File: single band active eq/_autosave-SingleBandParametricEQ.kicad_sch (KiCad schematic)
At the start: 18 parts, among them U1 TL081, U2 TL084

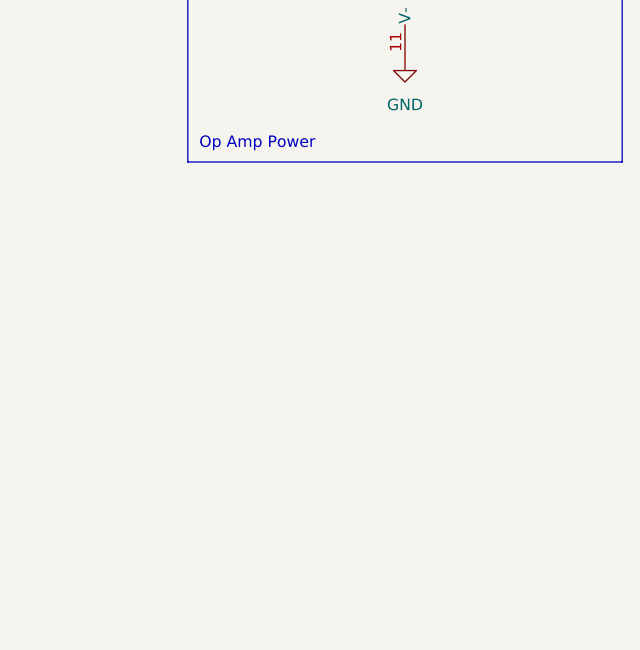
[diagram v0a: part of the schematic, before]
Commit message: Updated README
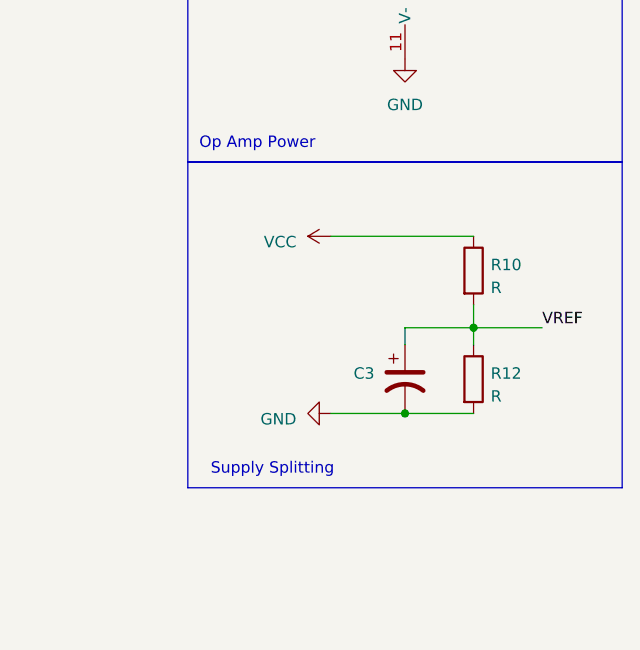
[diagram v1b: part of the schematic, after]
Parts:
- added C3: C_Polarized_US, symbol Device:C_Polarized_US
- added R10, R12: R, symbol Device:R
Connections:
- net GND: now also C3.2, R12.2
- net VCC: now also R10.1
- net VREF: now also C3.1, R10.2, R12.1
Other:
- note added: "Supply Splitting"
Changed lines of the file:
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@@
   (junction (at 53.975 46.99) (diameter 0) (color 0 0 0 0)
   )
+  (junction (at 268.605 69.85) (diameter 0) (color 0 0 0 0)
+  )
   (junction (at 173.99 54.61) (diameter 0) (color 0 0 0 0)
   )
@@
   (junction (at 43.18 124.46) (diameter 0) (color 0 0 0 0)
   )
+  (junction (at 260.985 79.375) (diameter 0) (color 0 0 0 0)
+  )
   (wire (pts (xy 66.04 63.5) (xy 112.395 63.5))
     (stroke (width 0) (type default))
@@
     (stroke (width 0) (type default))
   )
+  (wire (pts (xy 260.985 69.85) (xy 260.985 71.755))
+    (stroke (width 0) (type default))
+  )
   (wire (pts (xy 112.395 63.5) (xy 158.75 63.5))
     (stroke (width 0) (type default))
@@
     (stroke (width 0) (type default))
   )
+  (wire (pts (xy 260.985 69.85) (xy 268.605 69.85))
+    (stroke (width 0) (type default))
+  )
   (wire (pts (xy 92.71 41.91) (xy 92.71 49.53))
     (stroke (width 0) (type default))
@@
     (stroke (width 0) (type default))
   )
+  (wire (pts (xy 252.73 59.69) (xy 268.605 59.69))
+    (stroke (width 0) (type default))
+  )
   (wire (pts (xy 32.385 40.64) (xy 32.385 46.99))
     (stroke (width 0) (type default))
@@
     (stroke (width 0) (type default))
   )
+  (wire (pts (xy 260.985 79.375) (xy 268.605 79.375))
+    (stroke (width 0) (type default))
+  )
   (wire (pts (xy 76.2 111.76) (xy 76.2 127))
     (stroke (width 0) (type default))
@@
     (stroke (width 0) (type default))
   )
+  (wire (pts (xy 268.605 67.31) (xy 268.605 69.85))
+    (stroke (width 0) (type default))
+  )
   (wire (pts (xy 83.82 73.66) (xy 83.82 87.63))
     (stroke (width 0) (type default))
@@
     (stroke (width 0) (type default))
   )
+  (wire (pts (xy 268.605 69.85) (xy 276.225 69.85))
+    (stroke (width 0) (type default))
+  )
   (wire (pts (xy 101.6 85.09) (xy 104.14 85.09))
     (stroke (width 0) (type default))
@@
     (stroke (width 0) (type default))
   )
+  (wire (pts (xy 268.605 69.85) (xy 268.605 71.755))
+    (stroke (width 0) (type default))
+  )
   (wire (pts (xy 127.635 85.09) (xy 144.145 85.09))
     (stroke (width 0) (type default))
@@
     (stroke (width 0) (type default))
   )
+  (wire (pts (xy 260.985 79.375) (xy 252.73 79.375))
+    (stroke (width 0) (type default))
+  )
   (wire (pts (xy 137.16 52.07) (xy 138.43 52.07))
     (stroke (width 0) (type default))
@@
   )
   (rectangle (start 236.855 12.065) (end 285.115 51.435)
+    (stroke (width 0) (type default))
+    (fill (type none))
+  )
+  (rectangle (start 236.855 51.435) (end 285.115 87.63)
     (stroke (width 0) (type default))
     (fill (type none))
@@
   )
   (text "Cut/Boost Stage\n" (at 13.97 163.83 0)
+    (effects (font (size 1.27 1.27)) (justify left bottom))
+  )
+  (text "Supply Splitting\n" (at 239.395 86.36 0)
+    (effects (font (size 1.27 1.27)) (justify left bottom))
+  )
+  (label "VREF" (at 276.225 69.85 0) (fields_autoplaced)
     (effects (font (size 1.27 1.27)) (justify left bottom))
   )
@@
     )
   )
+  (symbol (lib_id "Device:R") (at 268.605 75.565 0) (unit 1)
+    (in_bom yes) (on_board yes) (dnp no) (fields_autoplaced)
+    (property "Reference" "R12" (at 270.51 74.93 0)
+      (effects (font (size 1.27 1.27)) (justify left))
+    )
+    (property "Value" "R" (at 270.51 77.47 0)
+      (effects (font (size 1.27 1.27)) (justify left))
+    )
+    (property "Footprint" "" (at 266.827 75.565 90)
+      (effects (font (size 1.27 1.27)) hide)
+    )
+    (property "Datasheet" "~" (at 268.605 75.565 0)
+      (effects (font (size 1.27 1.27)) hide)
+    )
+    (pin "1")
+    (pin "2")
+    (instances
+      (project "SingleBandParametricEQ"
+        (path "/3b2635d3-a197-4858-8292-d9ad69933c94"
+          (reference "R12") (unit 1)
+        )
+      )
+    )
+  )
   (symbol (lib_id "Device:R") (at 91.44 73.66 90) (unit 1)
     (in_bom yes) (on_board yes) (dnp no) (fields_autoplaced)
@@
     )
   )
+  (symbol (lib_id "Device:C_Polarized_US") (at 260.985 75.565 0) (unit 1)
+    (in_bom yes) (on_board yes) (dnp no)
+    (property "Reference" "C3" (at 255.27 74.93 0)
+      (effects (font (size 1.27 1.27)) (justify left))
+    )
+    (property "Value" "C_Polarized_US" (at 243.84 76.835 0)
+      (effects (font (size 1.27 1.27)) (justify left) hide)
+    )
+    (property "Footprint" "" (at 260.985 75.565 0)
+      (effects (font (size 1.27 1.27)) hide)
+    )
+    (property "Datasheet" "~" (at 260.985 75.565 0)
+      (effects (font (size 1.27 1.27)) hide)
+    )
+    (pin "1")
+    (pin "2")
+    (instances
+      (project "SingleBandParametricEQ"
+        (path "/3b2635d3-a197-4858-8292-d9ad69933c94"
+          (reference "C3") (unit 1)
+        )
+      )
+    )
+  )
   (symbol (lib_id "Device:R") (at 73.66 22.86 90) (unit 1)
     (in_bom yes) (on_board yes) (dnp no) (fields_autoplaced)
@@
     )
   )
+  (symbol (lib_id "power:VCC") (at 252.73 59.69 90) (unit 1)
+    (in_bom yes) (on_board yes) (dnp no) (fields_autoplaced)
+    (property "Reference" "#PWR03" (at 256.54 59.69 0)
+      (effects (font (size 1.27 1.27)) hide)
+    )
+    (property "Value" "VCC" (at 248.92 60.325 90)
+      (effects (font (size 1.27 1.27)) (justify left))
+    )
+    (property "Footprint" "" (at 252.73 59.69 0)
+      (effects (font (size 1.27 1.27)) hide)
+    )
+    (property "Datasheet" "" (at 252.73 59.69 0)
+      (effects (font (size 1.27 1.27)) hide)
+    )
+    (pin "1")
+    (instances
+      (project "SingleBandParametricEQ"
+        (path "/3b2635d3-a197-4858-8292-d9ad69933c94"
+          (reference "#PWR03") (unit 1)
+        )
+      )
+    )
+  )
   (symbol (lib_id "power:GND") (at 260.985 40.005 0) (unit 1)
     (in_bom yes) (on_board yes) (dnp no) (fields_autoplaced)
@@
         )
       )
+    )
+  )
+  (symbol (lib_id "power:GND") (at 252.73 79.375 270) (unit 1)
+    (in_bom yes) (on_board yes) (dnp no) (fields_autoplaced)
+    (property "Reference" "#PWR04" (at 246.38 79.375 0)
+      (effects (font (size 1.27 1.27)) hide)
+    )
+    (property "Value" "GND" (at 248.92 80.01 90)
+      (effects (font (size 1.27 1.27)) (justify right))
+    )
+    (property "Footprint" "" (at 252.73 79.375 0)
+      (effects (font (size 1.27 1.27)) hide)
+    )
+    (property "Datasheet" "" (at 252.73 79.375 0)
+      (effects (font (size 1.27 1.27)) hide)
+    )
+    (pin "1")
+    (instances
+      (project "SingleBandParametricEQ"
+        (path "/3b2635d3-a197-4858-8292-d9ad69933c94"
+          (reference "#PWR04") (unit 1)
+        )
+      )
+    )
+  )
+  (symbol (lib_id "Device:R") (at 268.605 63.5 0) (unit 1)
+    (in_bom yes) (on_board yes) (dnp no) (fields_autoplaced)
+    (property "Reference" "R10" (at 270.51 62.865 0)
+      (effects (font (size 1.27 1.27)) (justify left))
+    )
+    (property "Value" "R" (at 270.51 65.405 0)
+      (effects (font (size 1.27 1.27)) (justify left))
+    )
+    (property "Footprint" "" (at 266.827 63.5 90)
+      (effects (font (size 1.27 1.27)) hide)
+    )
+    (property "Datasheet" "~" (at 268.605 63.5 0)
+      (effects (font (size 1.27 1.27)) hide)
+    )
+    (pin "1")
+    (pin "2")
+    (instances
+      (project "SingleBandParametricEQ"
+        (path "/3b2635d3-a197-4858-8292-d9ad69933c94"
+          (reference "R10") (unit 1)
+        )
+      )
